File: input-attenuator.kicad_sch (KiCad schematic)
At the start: 110 parts, among them J1 DC_INTF, J3 RX_1_RF, J4 RX_2_RF, K1 EE2-5TNU-L, K2 EE2-5TNU-L, K3 EE2-5TNU-L, K4 EE2-5TNU-L, Q1 BC858, Q1 MMBT3904, Q2 BC858, Q2 MMBT3904, Q3 MMBT3904, Q4 MMBT3904, Q5 MMBT3904, Q6 MMBT3904, Q7 MMBT3904, Q8 MMBT3904, U1 74HC00

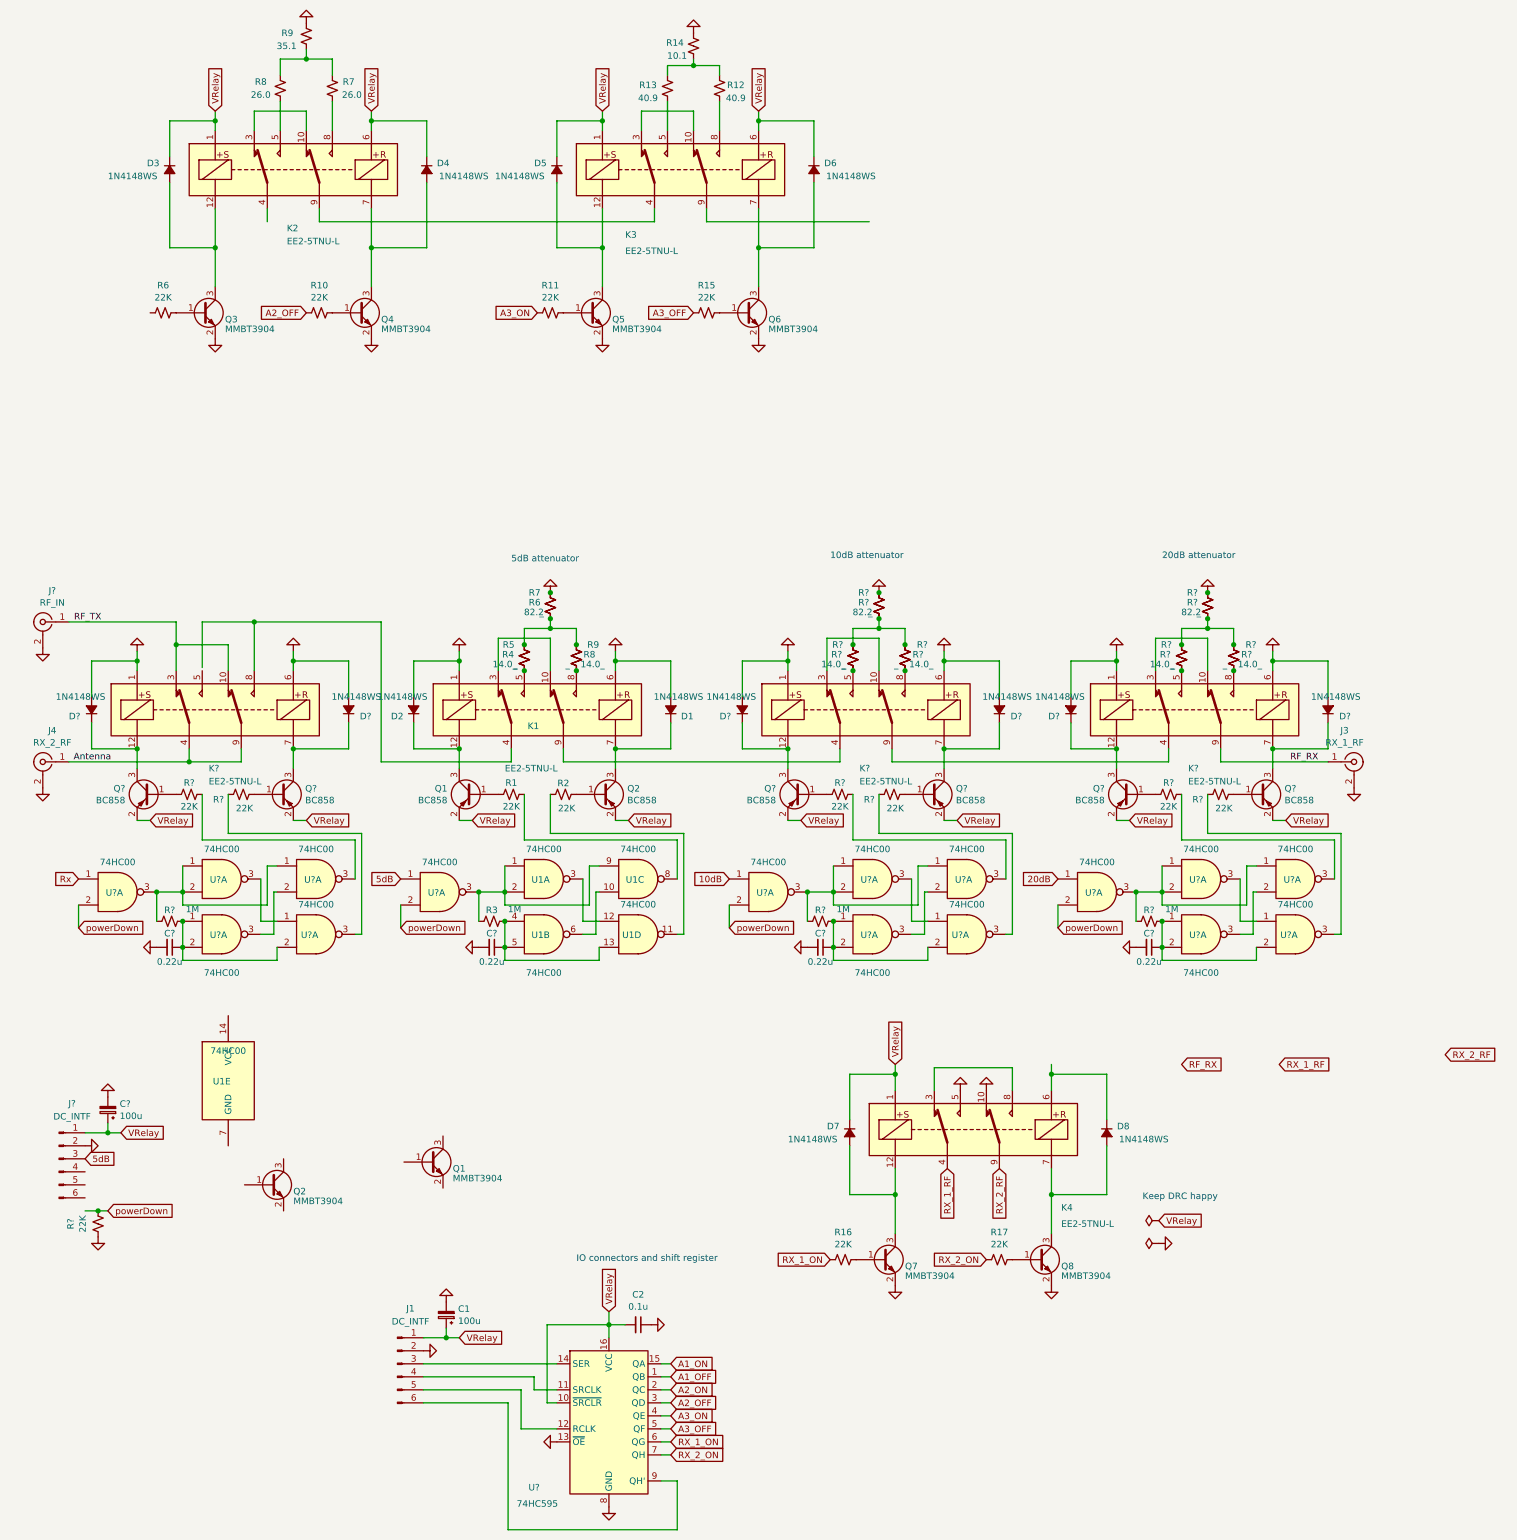
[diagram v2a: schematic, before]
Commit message: relaysPlaced
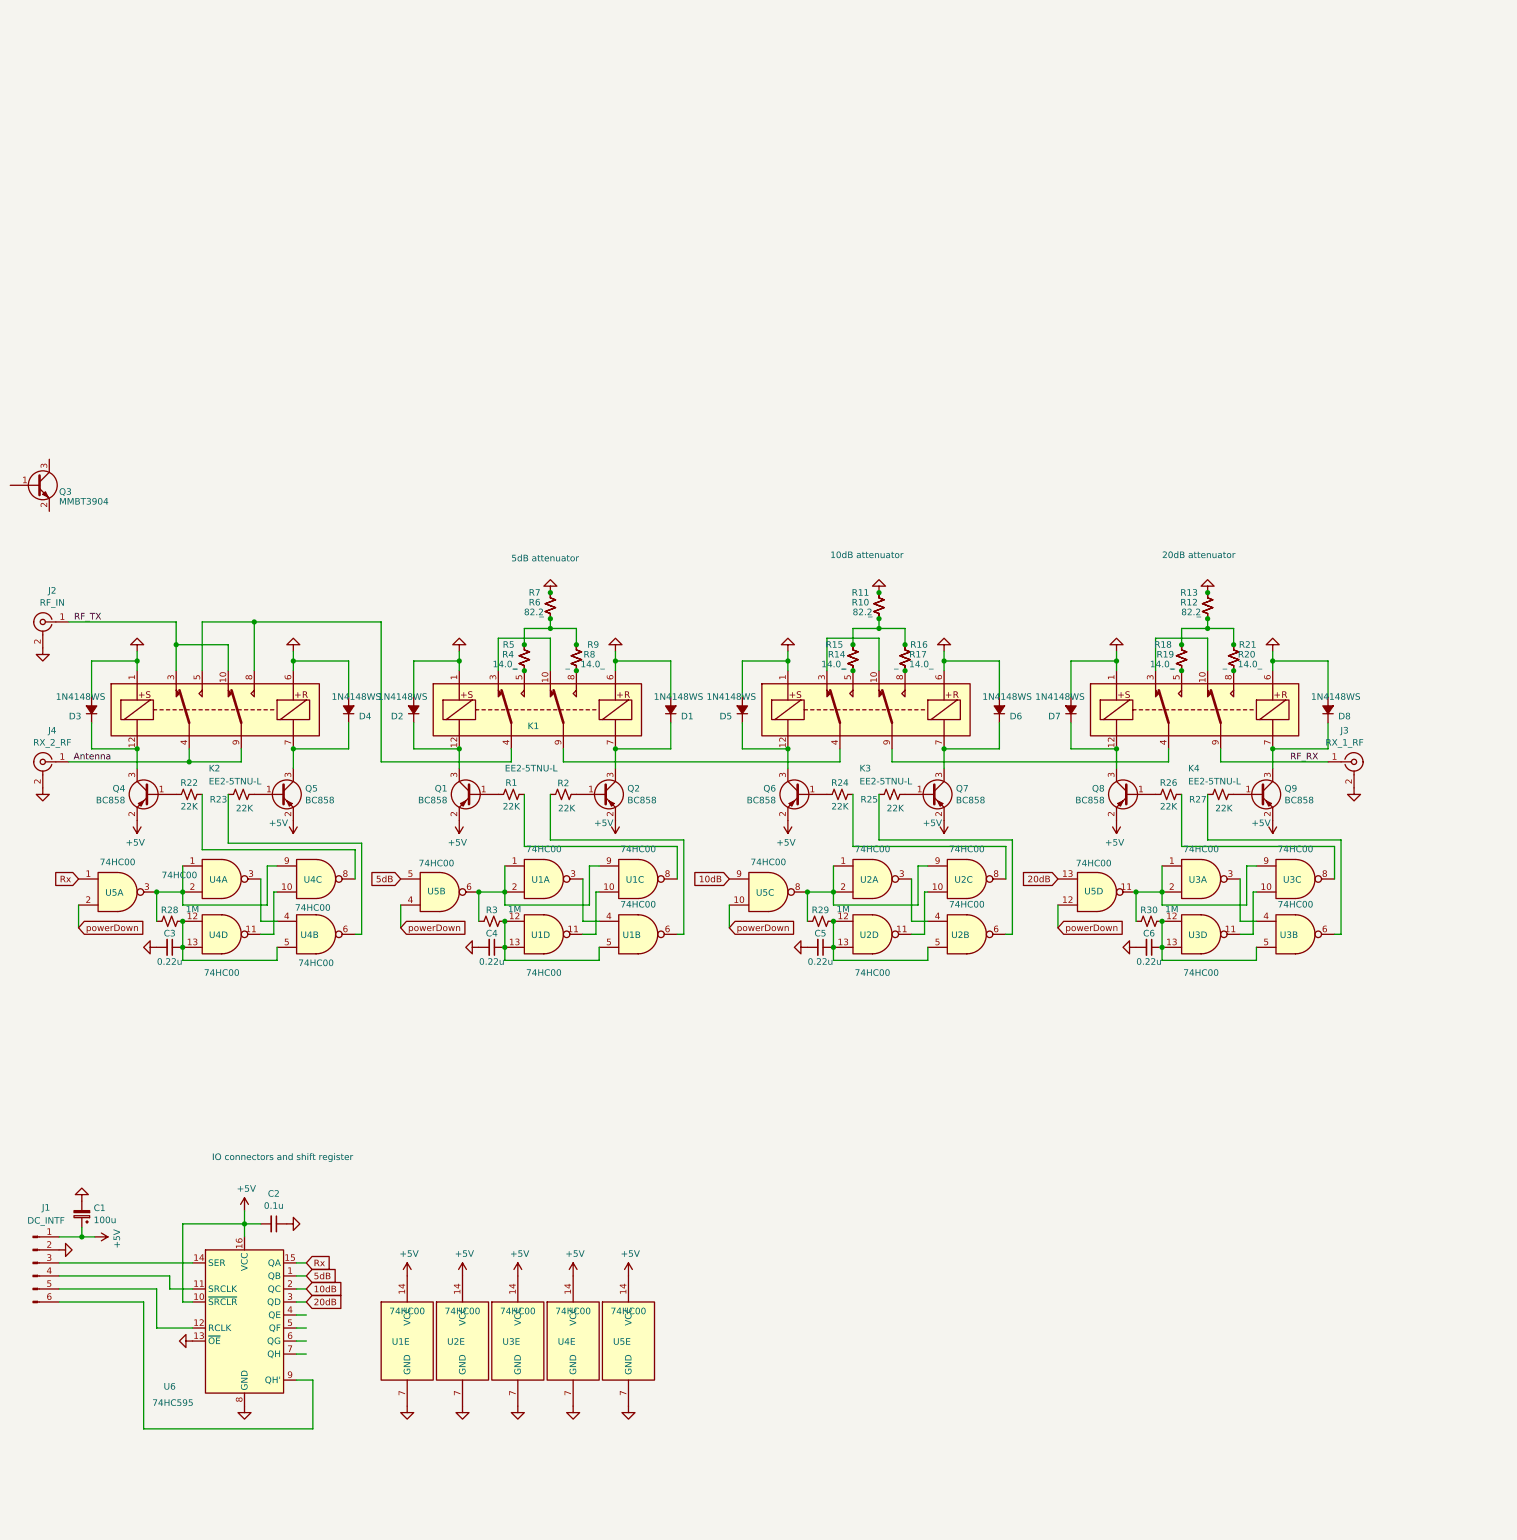
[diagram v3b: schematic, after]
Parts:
- removed C?: 100u, Capacitor_SMD:CP_Elec_6.3x5.4_Nichicon, symbol Device:CP_Small
- removed D3, D4, D5, D6, D7, D8: 1N4148WS, Diode_SMD:D_SOD-323, symbol Device:D_Small_ALT
- removed J?: DC_INTF, Connector_PinHeader_2.54mm:PinHeader_1x06_P2.54mm_Vertical, symbol Connector:Conn_01x06_Male
- removed K2, K3, K4: EE2-5TNU-L, Relay_SMD:Relay_DPDT_Kemet_EE2_NU_DoubleCoil, symbol Relay:EE2-5TNU
- removed Q2, Q3, Q4, Q5, Q6, Q7, Q8: MMBT3904, Package_TO_SOT_SMD:SOT-23, symbol Transistor_BJT:MMBT3904
- removed R10, R11, R15, R16, R17, R6, R?: 22K, Resistor_SMD:R_0805_2012Metric, symbol Device:R_Small_US
- removed R12, R13: 40.9, Resistor_SMD:R_0805_2012Metric, symbol Device:R_Small_US
- removed R14: 10.1, Resistor_SMD:R_0805_2012Metric, symbol Device:R_Small_US
- removed R7, R8: 26.0, Resistor_SMD:R_0805_2012Metric, symbol Device:R_Small_US
- removed R9: 35.1, Resistor_SMD:R_0805_2012Metric, symbol Device:R_Small_US
- added unit 5 of U2
- added unit 5 of U3
- added unit 5 of U4
- added unit 5 of U5
- U1: footprint (none) -> Package_SO:SO-14_3.9x8.65mm_P1.27mm
- U2, U3, U4, U5: renamed from U?; footprint (none) -> Package_SO:SO-14_3.9x8.65mm_P1.27mm
- gave numbers to parts that had none: 42
- renumbered Q1 to Q3
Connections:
- net A1_OFF is gone; now on net 5dB: U6.1 (QB)
- net A1_ON is gone; now on net Rx: U6.15 (QA)
- net A2_OFF is gone; now on net 20dB: U6.3 (QD)
- net A2_ON is gone; now on net 10dB: U6.2 (QC)
- net VRelay is gone; now on net +5V: C1.1, C2.2, J1.1 (Pin_1), Q1.2 (E), Q2.2 (E), Q4.2 (E), Q5.2 (E), Q6.2 (E), Q7.2 (E), Q8.2 (E), Q9.2 (E), U6.10 (~SRCLR), U6.16 (VCC)
- net 10dB: now also U5.9; no longer U5.1
- net 20dB: now also U5.13; no longer U5.1
- net 5dB: now also U5.5; no longer U5.1
- net GND: now also U1.7 (GND), U2.7 (GND), U3.7 (GND), U4.7 (GND), U5.7 (GND)
- net powerDown: now also U5.10, U5.12, U5.4; no longer U5.2, U5.2, U5.2
- net at K1.4, K2.8: now also K2.5
- net at R2.1: now also U1.6; no longer U1.11
- net at R27.1: now also U3.6; no longer U3.3
- net at R3.1, U1.1, U1.2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: now also U5.6; no longer U5.3
- net at U1.3: now also U1.4; no longer U1.12
- net at U2.3: now also U2.4; no longer U2.1
- net at R25.1: now also U2.6; no longer U2.3
- net at R30.1, U3.1, U3.2: now also U3.9, U5.11; no longer U3.1, U5.3
- net at R28.1, U4.1, U4.2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: now also U4.9; no longer U4.1
- net at R26.1: now also U3.8; no longer U3.3
- net at U1.10: now also U1.11; no longer U1.6
- net at R22.1: now also U4.8; no longer U4.3
- net +5V: now reaches U1.14 (VCC)
- net +5V: now also U2.14 (VCC), U3.14 (VCC), U4.14 (VCC), U5.14 (VCC)
- net at R29.1, U2.1, U2.2: now also U2.9, U5.8; no longer U2.1, U5.3
- net at R23.1: now also U4.6; no longer U4.3
- net at R24.1: now also U2.8; no longer U2.3
- net at U3.3: now also U3.4; no longer U3.1
- net at U4.3: now also U4.4; no longer U4.1
- net A3_OFF: no longer names the net of U6.5 (QF)
- net A3_ON: no longer names the net of U6.4 (QE)
- net RX_1_ON: no longer names the net of U6.6 (QG)
- net RX_2_ON: no longer names the net of U6.7 (QH)
- new net: C4.1, R3.2, U1.12, U1.13, U1.5
- new net: C5.1, R29.2, U2.12, U2.13, U2.5
- new net: C6.1, R30.2, U3.12, U3.13, U3.5
- new net: U3.10, U3.11
- new net: U4.10, U4.11
- new net: U2.10, U2.11
- new net: C3.1, R28.2, U4.12, U4.13, U4.5
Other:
- note removed: "Keep DRC happy"
- moved on the sheet: C1, C2, J1, Q3, U1E, U6
